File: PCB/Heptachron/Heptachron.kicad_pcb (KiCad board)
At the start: 2 copper layers, 42 x 25 mm, 48 parts, among them IC1 BQ25185DLHR, J1 5V, J2 GND, J3 UPDI, J4 BAT+, J5 BAT-, Q1 Q_PH, SW1 SW_Push, SW2 SW_Push, U7 IS31FL3729, U8 ATtiny424-SS, X1 RV-3028-C7

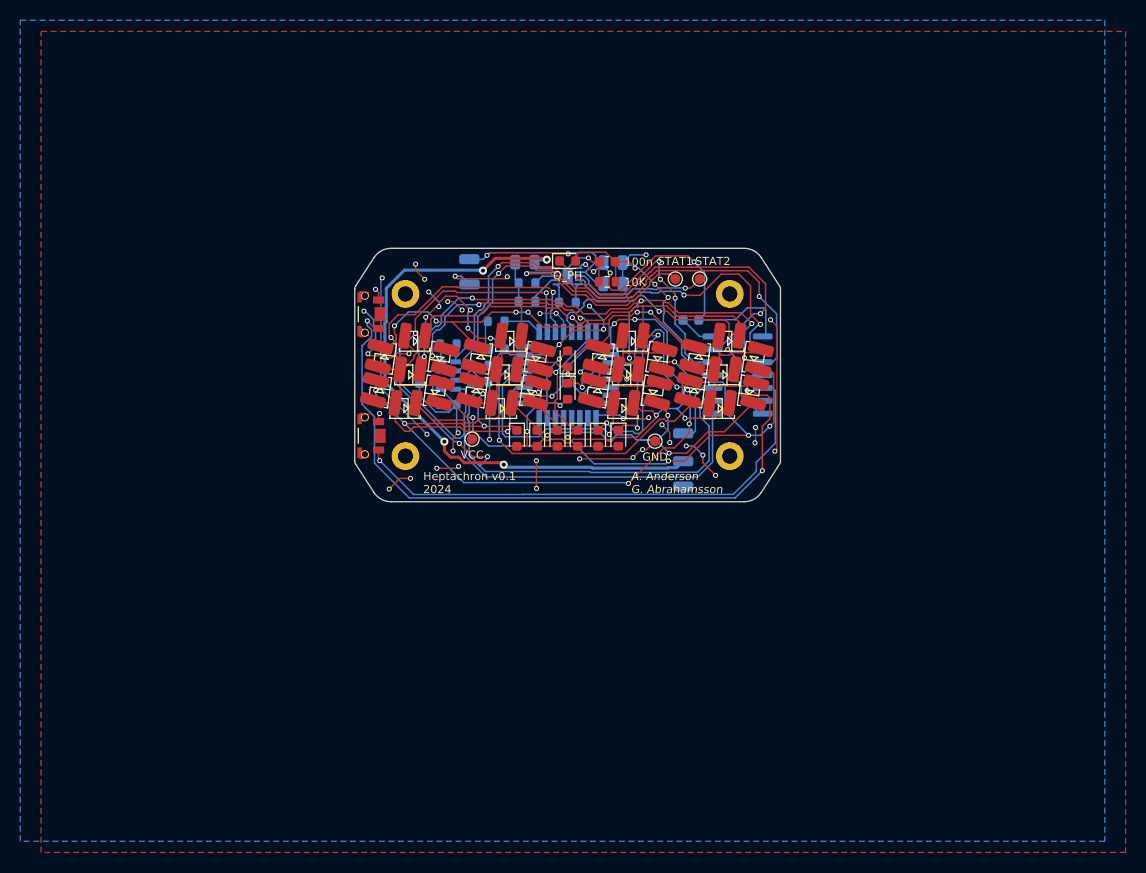
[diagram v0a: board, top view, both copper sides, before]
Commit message: PCB v0.2
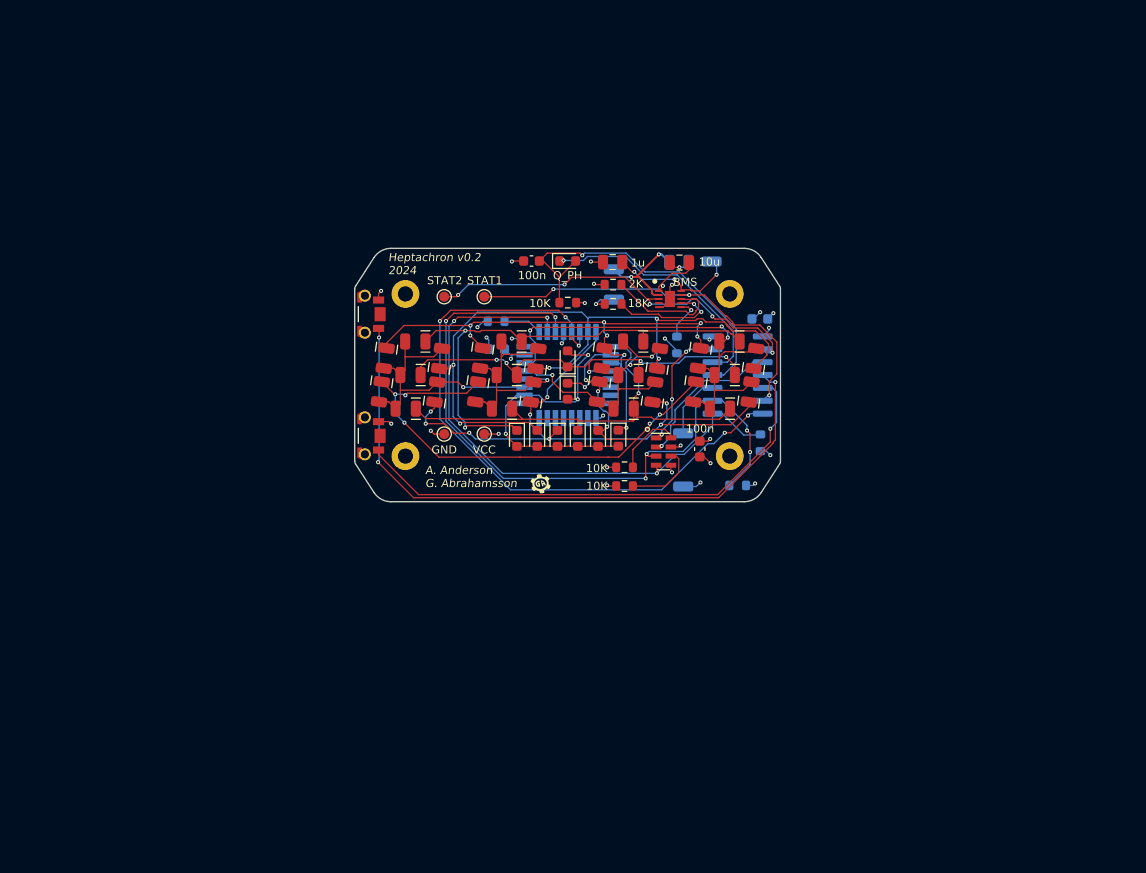
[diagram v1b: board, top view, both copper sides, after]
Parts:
- C1, C8, C9, IC1, R1, R17, R18, R2, X1: moved to F.Cu
- U1, U2, U3, U4: footprint Heptachron-Lib:7-segment-digit-Cree -> Heptachron-Lib:7-SEGMENT_NEW
- moved C1 28.6 mm to (161.0, 108.3)
- moved R13 28.3 mm to (167.0, 107.7), turned to 90 degrees
- moved R14 28.0 mm to (164.8, 111.9)
- moved TP2 25.3 mm to (135.8, 93.3)
- moved X1 22.5 mm to (157.5, 108.5)
- moved R2 21.2 mm to (153.6, 110.1), turned to 0 degrees
- moved TP6 20.8 mm to (135.8, 106.8)
- moved J1 19.9 mm to (162.2, 89.8)
- moved R1 19.2 mm to (153.6, 112.0), turned to 0 degrees
- moved TP1 18.9 mm to (139.8, 93.3)
- moved J5 14.3 mm to (152.6, 93.6)
- moved J4 14.3 mm to (152.6, 90.6)
- moved R19 11.6 mm to (158.8, 98.0), turned to 90 degrees
- moved IC1 10.3 mm to (158.1, 93.5), turned to 0 degrees
- moved C8 8.66 mm to (152.4, 89.9)
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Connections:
- D37 pad 1: /CS6 -> /CS8
- U7 pad 5: unconnected-(U7-CS8-Pad5) -> /CS8
- U8 pad 2: //CE -> /STAT2
- U8 pad 6: unconnected-(U8-PB3-Pad6) -> /STAT1
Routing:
- net VCC: track 108.4 -> 16.0 mm, vias 18 -> 9
- net GND: track 93.4 -> 31.2 mm, vias 35 -> 23
- net +5V: track 64.0 -> 13.1 mm, vias 4 -> 3
- net /RTC_CLK: track 50.6 -> 12.6 mm, vias 2 -> 3
- net /RTC_INT: track 50.8 -> 15.3 mm, vias 2 -> 1
- net /LED_EN: track 30.6 -> 62.4 mm, vias 2 -> 4
- net //CE: track 27.9 -> 0.00 mm, vias 2 -> 0
- net /CS7: track 68.9 -> 41.1 mm, vias 8 -> 5
- net /STAT2: track 13.5 -> 39.8 mm, vias 1 -> 5
- net /STAT1: track 20.6 -> 38.7 mm, vias 1 -> 3
- net /CS5: track 80.7 -> 63.5 mm, vias 9 -> 8
- net /SCL: track 86.4 -> 70.4 mm, vias 4 -> 6
- net /SDA: track 74.0 -> 58.5 mm, vias 2 -> 3
- net /SW2: track 42.2 -> 28.9 mm, vias 1 -> 3
- net /CS4: track 57.0 -> 44.5 mm, vias 4 -> 1
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- added copper zone on In1.Cu, net GND
- added copper zone on In2.Cu, net VCC
- removed copper zone on B.Cu, net GND
- removed copper zone on F.Cu, net VCC
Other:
- copper layers 2 -> 4
- board text added: "Heptachron v0.2 2024"
- board text removed: "Heptachron v0.1 2024"
